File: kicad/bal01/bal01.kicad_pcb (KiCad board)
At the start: 2 copper layers, 25 x 25 mm, 9 parts, among them IC1 AS5601-ASOT

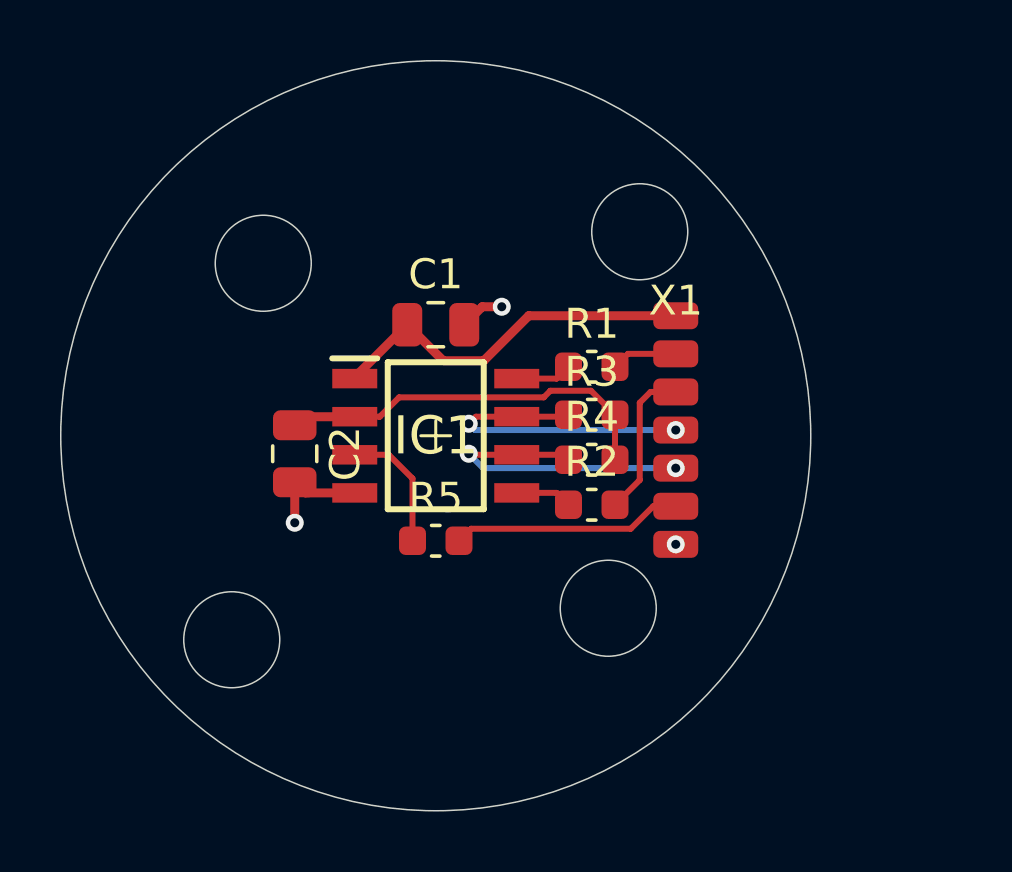
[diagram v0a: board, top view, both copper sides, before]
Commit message: bal01 olmost finished
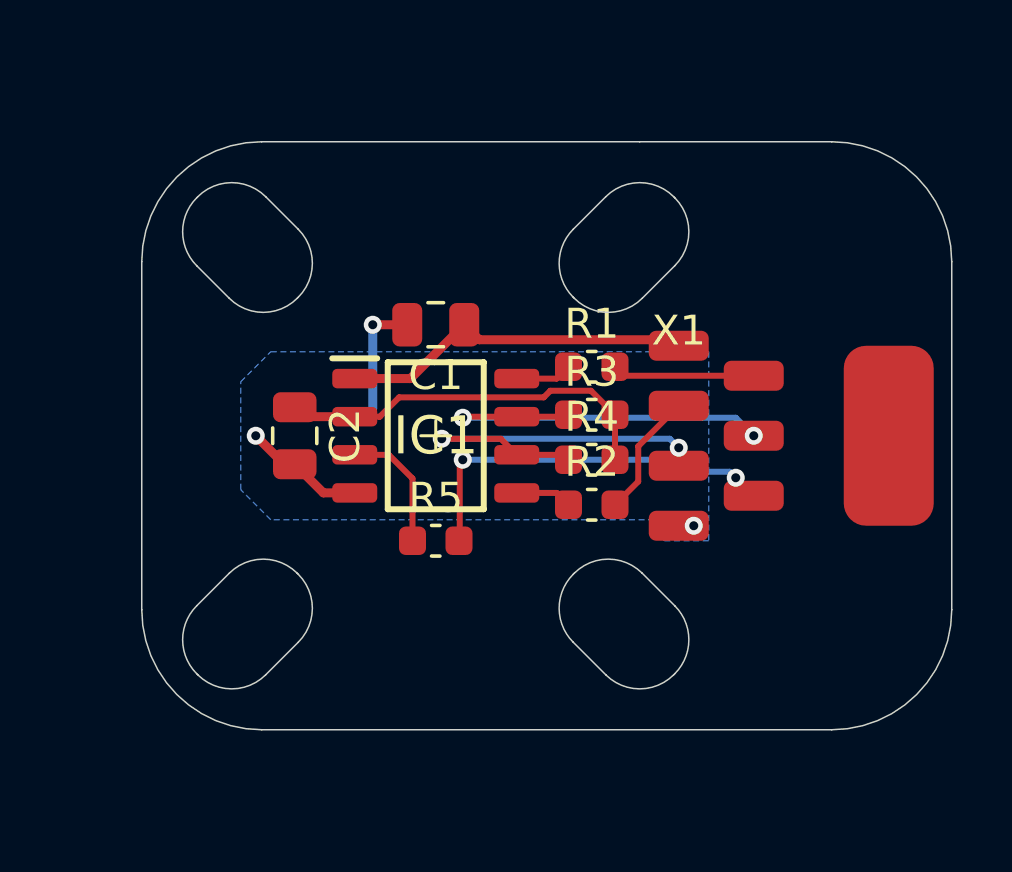
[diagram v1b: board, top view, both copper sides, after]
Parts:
- X1: footprint bal:H7_Pads_1.27mm -> bal:H7_Pads_1.27mm-001
- moved X1 1.00 mm to (138.1, 97.0)
- moved C2 0.60 mm to (125.3, 100.0)
- turned C1 to 180 degrees
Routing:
- net PUSH: track 7.70 -> 12.9 mm, vias 0 -> 2
- net SCL: track 10.4 -> 13.5 mm
- net GND: track 5.00 -> 8.04 mm
- net SDA: track 10.5 -> 13.1 mm
- net A: track 2.20 -> 4.75 mm
- net B: track 5.09 -> 4.18 mm
- net +5V: track 12.6 -> 11.9 mm
- added copper zone on B.Cu, net GND
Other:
- board size 25 x 25 mm -> 27 x 19.6 mm
